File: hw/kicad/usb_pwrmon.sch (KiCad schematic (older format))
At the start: 4 parts

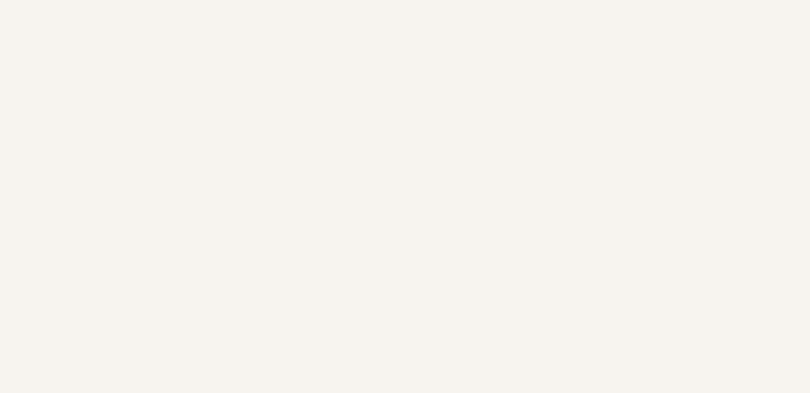
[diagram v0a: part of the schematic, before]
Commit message: - add shunt
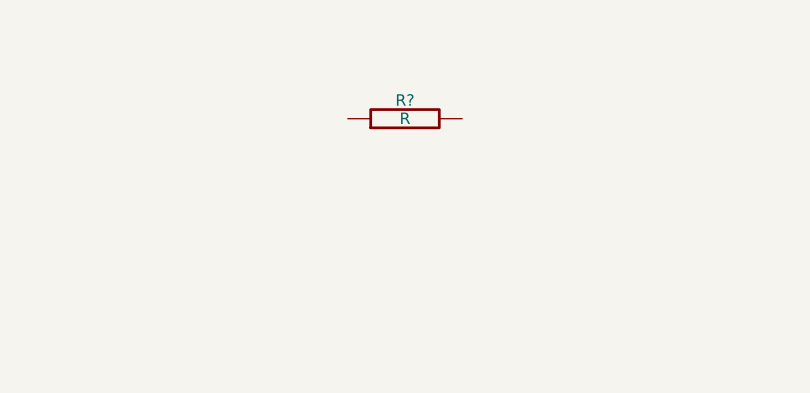
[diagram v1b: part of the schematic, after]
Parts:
- added R?: R, symbol R
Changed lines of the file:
@@
-EESchema Schematic File Version 2  date 2/22/2013 6:04:26 PM
+EESchema Schematic File Version 2  date 2/22/2013 6:14:41 PM
 LIBS:power
 LIBS:device
@@
 $EndDescr
 $Comp
+L R R?
+U 1 1 5127FAE0
+P 5900 2550
+F 0 "R?" V 5980 2550 50  0000 C CNN
+F 1 "R" V 5900 2550 50  0000 C CNN
+	1    5900 2550
+	0    -1   -1   0
+$EndComp
+$Comp
 L USB_NP_1 J?
